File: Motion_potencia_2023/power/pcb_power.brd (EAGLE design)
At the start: 95 x 95 mm, 0 parts

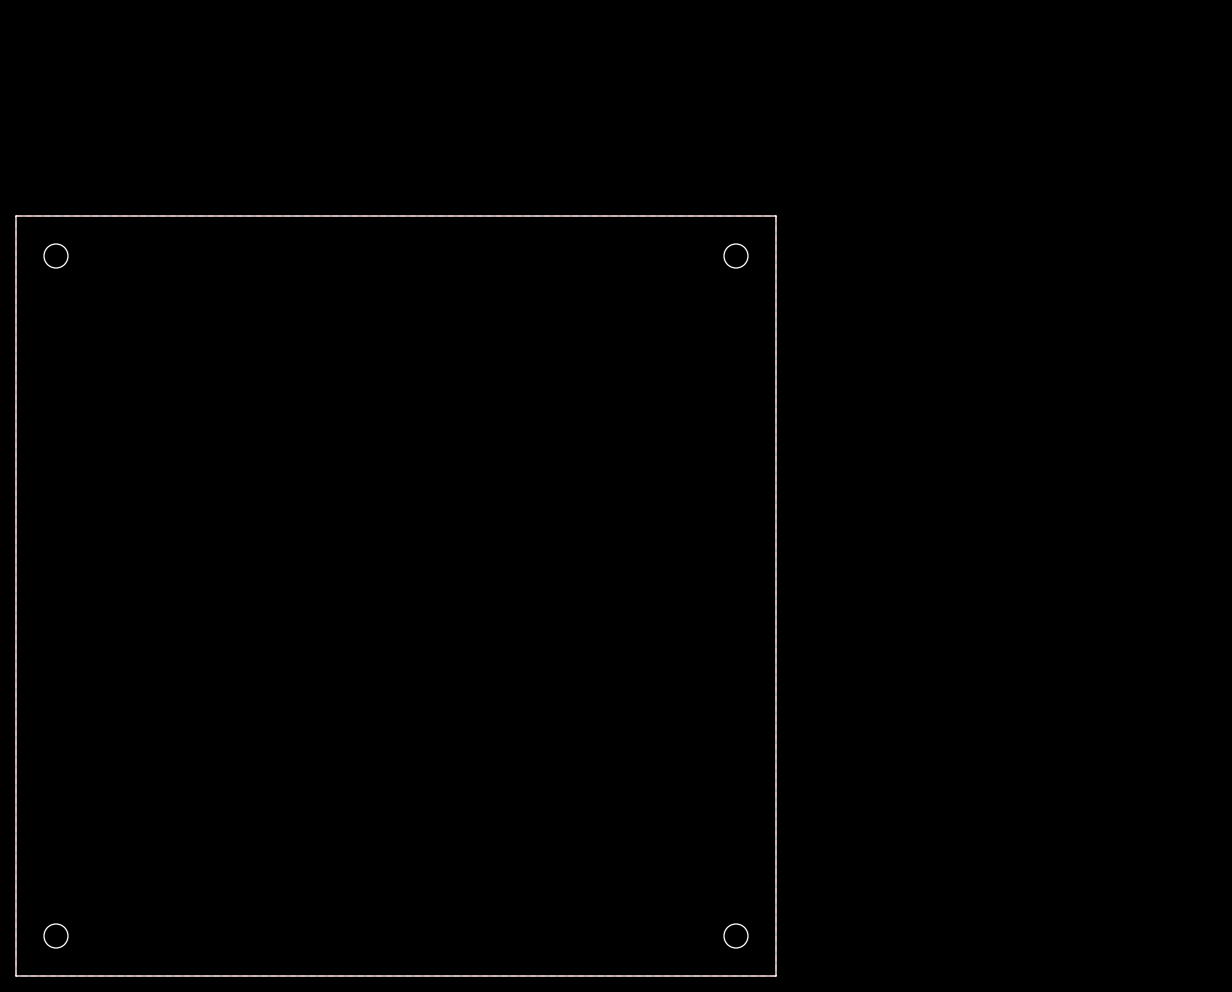
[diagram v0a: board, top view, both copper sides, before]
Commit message: main, power
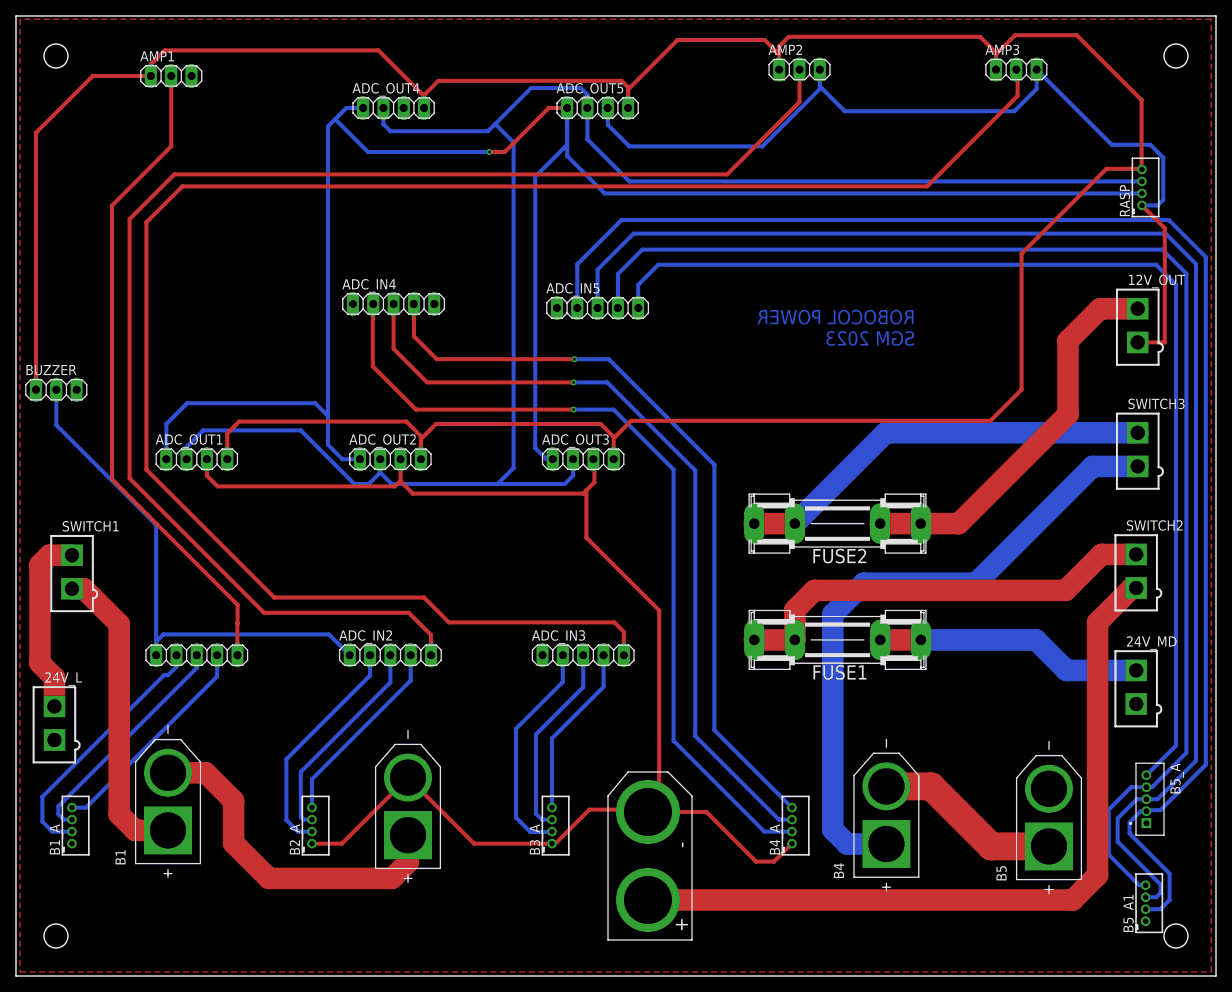
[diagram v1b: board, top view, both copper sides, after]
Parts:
- added 12V_OUT, 24V_L, 24V_MD, SWITCH1, SWITCH2, SWITCH3: 5566-25569-2, molex_arreglado_2:5569-2
- added ADC_IN1, ADC_IN2, ADC_IN3, ADC_IN4, ADC_IN5: (no value), pinhead:1X05
- added ADC_OUT1, ADC_OUT2, ADC_OUT3, ADC_OUT4, ADC_OUT5: (no value), pinhead:1X04
- added AMP1, AMP2, AMP3, BUZZER: (no value), pinhead:1X03
- added B1, B2, B4, B5: XT60-M, XT60-M:AMASS_XT60-M
- added B1_A, B2_A, B3_A, B4_A, B5_A1, RASP: B4B-ZR, con-jst:B4B-ZR
- added B3: XT90, Robocol_Eagle_Libraries:XT90_PADS
- added B5_A: B5B-ZR(LF)(SN), B5B-ZR_LF__SN_:JST_B5B-ZR(LF)(SN)
- added FUSE1, FUSE2: (no value), fuse:SHK20L
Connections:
- new net 5V: ADC_OUT1.4, ADC_OUT2.4, ADC_OUT3.4, ADC_OUT4.4, ADC_OUT5.4, AMP1.1, AMP2.1, AMP3.1, BUZZER.1, RASP.4
- new net AI1: ADC_IN1.2, B1_A.2
- new net AI10: ADC_IN3.3, B3_A.3
- new net AI11: ADC_IN3.4, B3_A.4
- new net AI12: ADC_IN3.5, AMP3.2
- new net AI13: ADC_IN4.2, B4_A.2
- new net AI14: ADC_IN4.3, B4_A.3
- new net AI15: ADC_IN4.4, B4_A.4
- new net AI16: ADC_IN4.5
- new net AI17: ADC_IN5.2, B5_A.2, B5_A1.2
- new net AI18: ADC_IN5.3, B5_A.3, B5_A1.3
- new net AI19: ADC_IN5.4, B5_A.4, B5_A1.4
- new net AI2: ADC_IN1.3, B1_A.3
- new net AI20: ADC_IN5.5, B5_A.5
- new net AI3: ADC_IN1.4, B1_A.4
- new net AI4: ADC_IN1.5, AMP1.2
- new net AI5: ADC_IN2.2, B2_A.2
- new net AI6: ADC_IN2.3, B2_A.3
- new net AI7: ADC_IN2.4, B2_A.4
- new net AI8: ADC_IN2.5, AMP2.2
- new net AI9: ADC_IN3.2, B3_A.2
- new net AO1: ADC_IN1.1, ADC_IN2.1, BUZZER.2
- new net GND: 12V_OUT.1, 24V_L.1, 24V_MD.1, ADC_OUT1.3, ADC_OUT2.3, ADC_OUT3.3, ADC_OUT4.3, ADC_OUT5.3, AMP1.3, AMP2.3, AMP3.3, B1_A.1, B2.N, B2_A.1, B3.GND, B3_A.1, B4_A.1, B5.N, B5_A.1, B5_A1.1, BUZZER.3, RASP.1
- new net N$12: 24V_MD.2, FUSE1.1A, FUSE1.1B
- new net N$13: FUSE1.2A, FUSE1.2B, SWITCH2.2
- new net N$14: 12V_OUT.2, FUSE2.1A, FUSE2.1B
- new net N$15: FUSE2.2A, FUSE2.2B, SWITCH3.2
- new net N$16: 24V_L.2, SWITCH1.2
- new net N$17: B1.N, B2.P
- new net N$20: B4.N, B5.P
- new net SCL: ADC_OUT1.1, ADC_OUT2.1, ADC_OUT3.1, ADC_OUT4.1, ADC_OUT5.1, RASP.2
- new net SDAT: ADC_OUT1.2, ADC_OUT2.2, ADC_OUT3.2, ADC_OUT4.2, ADC_OUT5.2, RASP.3
- new net SWITCH1-1: B1.P, SWITCH1.1
- new net SWITCH2-1: B3.VCC, SWITCH2.1
- new net SWITCH3-1: B4.P, SWITCH3.1
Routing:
- net 5V: track 0.00 -> 361.4 mm
- net GND: track 0.00 -> 294.7 mm
- net SCL: track 0.00 -> 235.9 mm, vias 0 -> 1
- net AI12: track 0.00 -> 220.7 mm
- net SDAT: track 0.00 -> 213.2 mm
- net AI17: track 0.00 -> 179.5 mm
- net AI8: track 0.00 -> 174.6 mm
- net AI18: track 0.00 -> 171.6 mm
- net AI19: track 0.00 -> 162.2 mm
- net AI20: track 0.00 -> 135.0 mm
- net AI13: track 0.00 -> 104.2 mm, vias 0 -> 1
- net AI14: track 0.00 -> 99.2 mm, vias 0 -> 1
- net SWITCH2-1: track 0.00 -> 95.7 mm
- net AI15: track 0.00 -> 95.1 mm, vias 0 -> 1
- net AI4: track 0.00 -> 82.0 mm
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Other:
- board size 95 x 95 mm -> 150 x 120 mm
- board text added: "ROBOCOL POWER SGM 2023"
